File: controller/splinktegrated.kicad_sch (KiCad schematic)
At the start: 41 parts, among them J1 USB_C_Receptacle_USB2.0, J11 Conn_01x07_Socket, J5 Conn_01x02, J7 Cirque, SW2 NA_SW_SPST, U1 RP2040, U3 XC6210B332MR-G, U4 USBLC6-2P6, U5 W25Q128JVS, Y1 Crystal_GND24

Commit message: work
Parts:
- J11: footprint Connector_PinSocket_2.54mm:PinSocket_1x07_P2.54mm_Vertical -> Library:PinSocket_1x07_P2.54mm_Vertical
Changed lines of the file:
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@@
 			)
 		)
-		(property "Footprint" "Connector_PinSocket_2.54mm:PinSocket_1x07_P2.54mm_Vertical"
+		(property "Footprint" "Library:PinSocket_1x07_P2.54mm_Vertical"
 			(at 304.8 40.64 0)
 			(effects

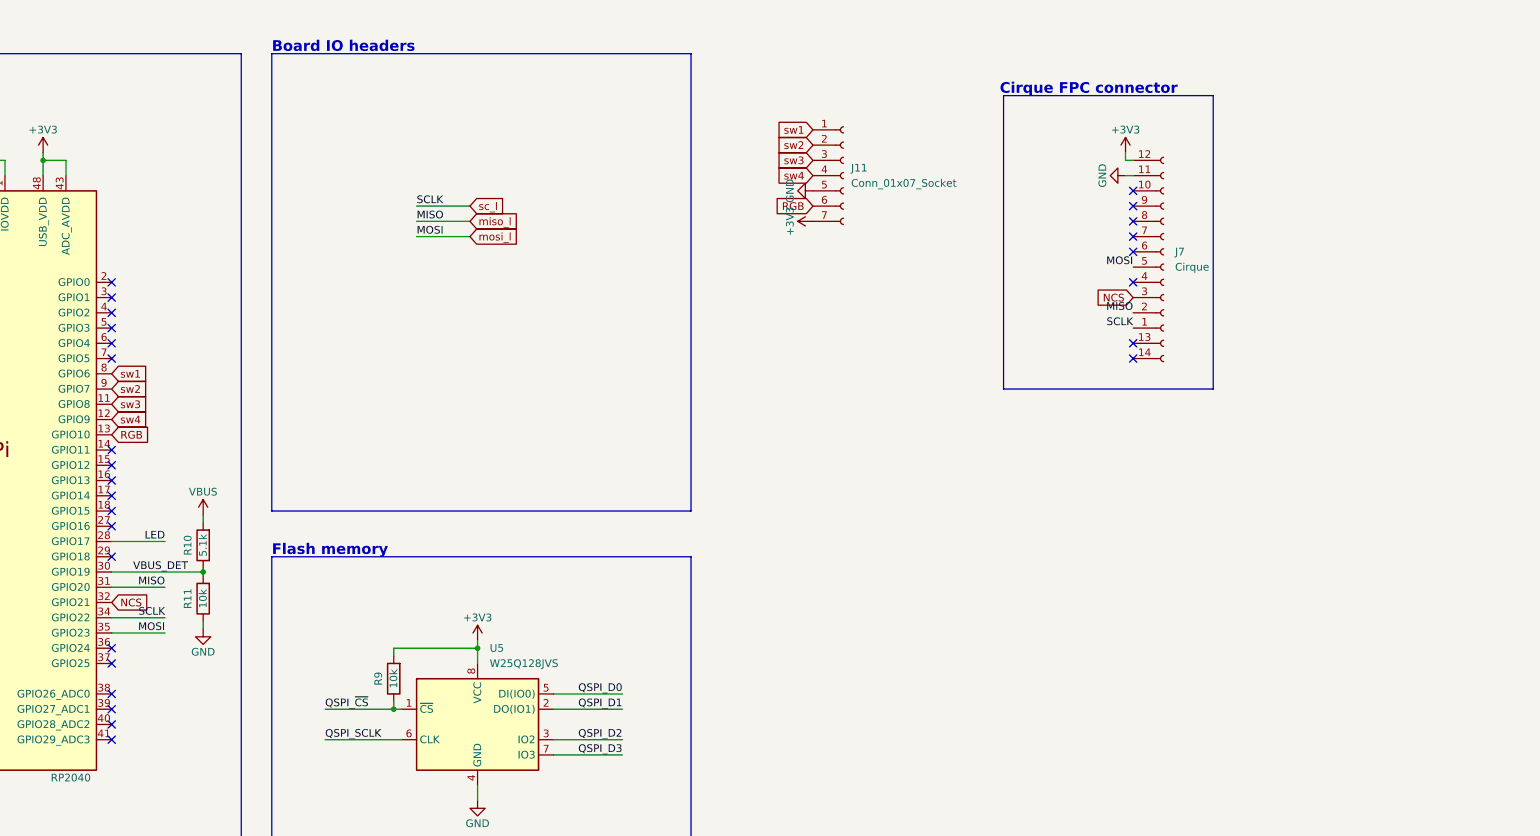
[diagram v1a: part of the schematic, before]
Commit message: VIK
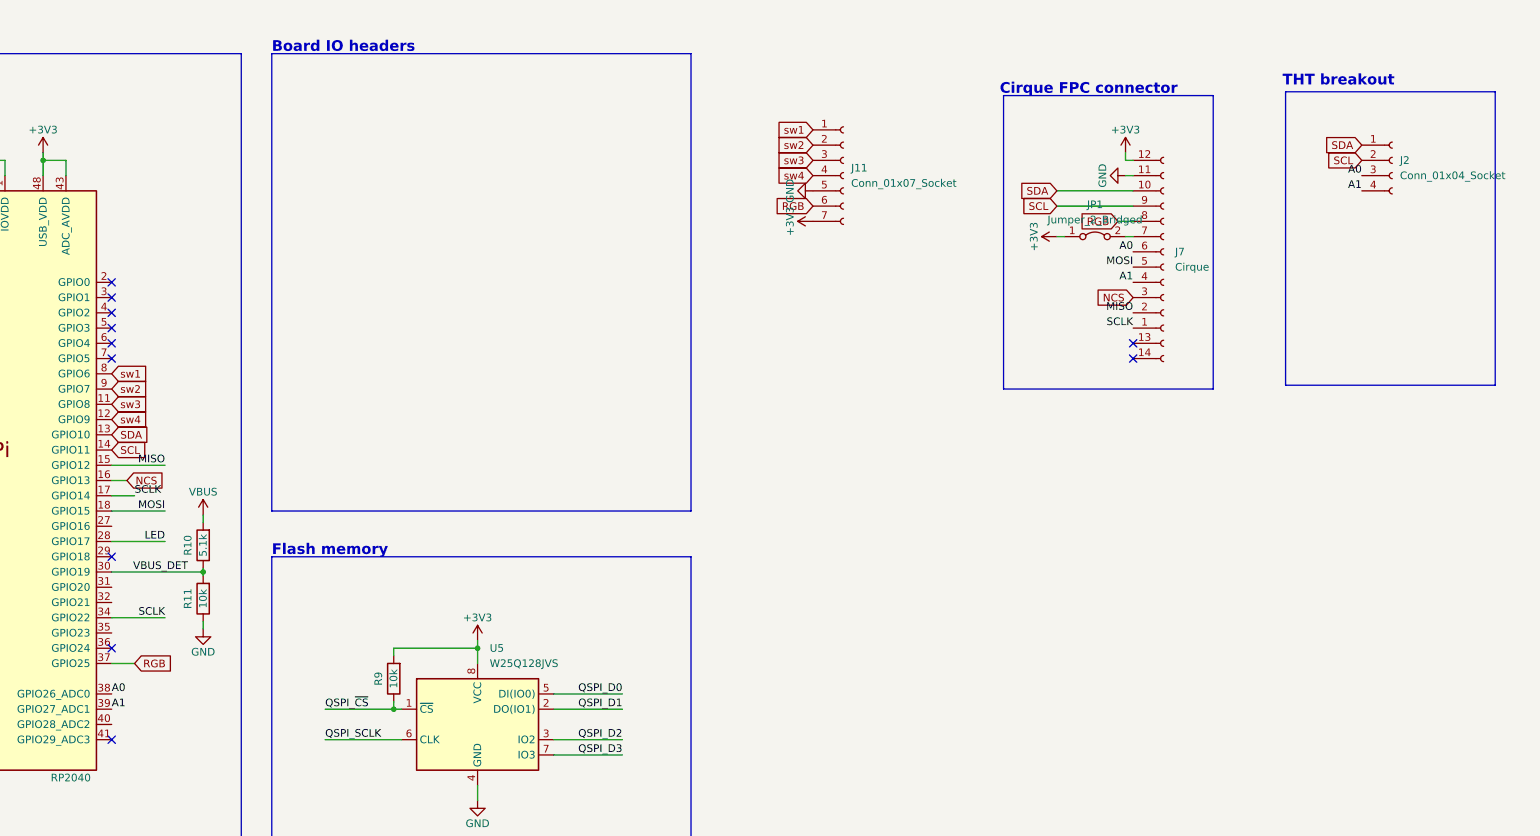
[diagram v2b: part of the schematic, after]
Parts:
- added J2: Conn_01x04_Socket, Connector_PinSocket_2.54mm:PinSocket_1x04_P2.54mm_Vertical, symbol Connector:Conn_01x04_Socket
- added JP1: Jumper_2_Bridged, Jumper:SolderJumper-2_P1.3mm_Open_RoundedPad1.0x1.5mm, symbol Jumper:Jumper_2_Bridged
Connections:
- net sc_l is gone; now on net SCLK: J7.1 (Pin_1), U1.34 (GPIO22)
- net +3V3: now also JP1.1 (A)
- net NCS: now also U1.16 (GPIO13); no longer U1.32 (GPIO21)
- net RGB: now also J7.8 (Pin_8), U1.37 (GPIO25); no longer U1.13 (GPIO10)
- net SCL: now reaches U1.14 (GPIO11)
- net SCL: now also J7.9 (Pin_9), J2.2 (Pin_2)
- net MISO: now reaches U1.15 (GPIO12)
- net MISO: now also J7.2 (Pin_2)
- net SCLK: now reaches U1.17 (GPIO14)
- net MOSI: now reaches U1.18 (GPIO15)
- net MOSI: now also J7.5 (Pin_5)
- net A0: now reaches U1.38 (GPIO26_ADC0)
- net A0: now also J7.6 (Pin_6), J2.3 (Pin_3)
- net A1: now reaches U1.39 (GPIO27_ADC1)
- net A1: now also J7.4 (Pin_4), J2.4 (Pin_4)
- net SDA: now reaches J7.10 (Pin_10)
- net SDA: now also U1.13 (GPIO10), J2.1 (Pin_1)
- net at J7.7 (Pin_7): now also JP1.2 (B)
- net miso_l: no longer names the net of U1.31 (GPIO20)
- net miso_l: no longer J7.2 (Pin_2)
- net mosi_l: no longer names the net of U1.35 (GPIO23)
- net mosi_l: no longer J7.5 (Pin_5)
- no-connect marks 31 -> 15
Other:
- note added: "THT breakout"
